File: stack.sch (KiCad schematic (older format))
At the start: 6 parts, among them U26 74LS245, U27 74LS173, U28 74LS173, U29 74LS245, U30 74LS173, U31 74LS173

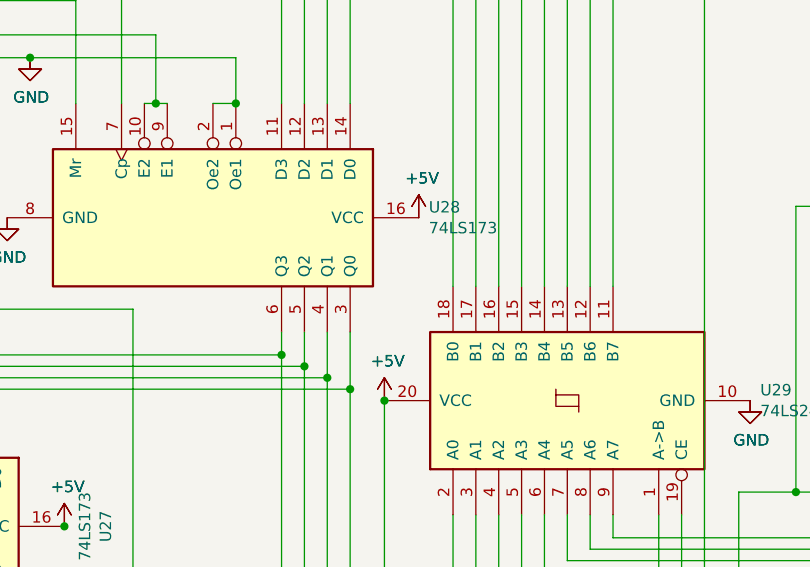
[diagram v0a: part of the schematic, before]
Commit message: fixed more errors
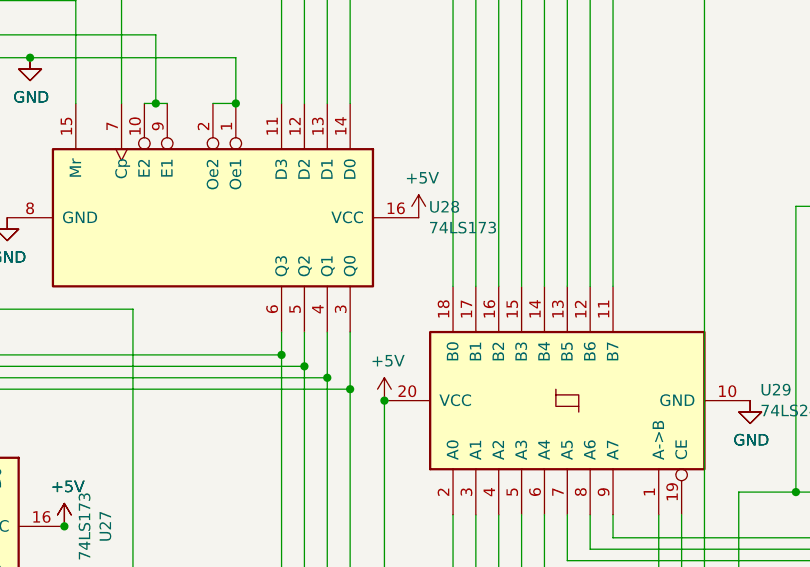
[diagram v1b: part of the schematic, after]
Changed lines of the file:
@@
-$Comp
-L 16bitCpu-rescue:+5V-power #PWR?
-U 1 1 616C3797
-P 5800 4300
-AR Path="/616C3797" Ref="#PWR?"  Part="1"
-AR Path="/5F67C726/616C3797" Ref="#PWR?"  Part="1"
-AR Path="/5F70885A/616C3797" Ref="#PWR?"  Part="1"
-AR Path="/5F733C5E/616C3797" Ref="#PWR?"  Part="1"
-AR Path="/602D4838/616C3797" Ref="#PWR?"  Part="1"
-AR Path="/603B00C8/616C3797" Ref="#PWR?"  Part="1"
-AR Path="/603B766D/616C3797" Ref="#PWR?"  Part="1"
-AR Path="/5F74778C/616C3797" Ref="#PWR?"  Part="1"
-AR Path="/5FB94562/616C3797" Ref="#PWR?"  Part="1"
-AR Path="/61968B9B/616C3797" Ref="#PWR0110"  Part="1"
-F 0 "#PWR0110" H 5800 4150 50  0001 C CNN
-F 1 "+5V" H 5815 4473 50  0000 C CNN
-F 2 "" H 5800 4300 50  0001 C CNN
-F 3 "" H 5800 4300 50  0001 C CNN
-	1    5800 4300
-	1    0    0    -1
-$EndComp
 $Comp
 L 16bitCpu-rescue:+5V-power #PWR?
@@
 	1    0    0    -1
 $EndComp
-$Comp
-L 16bitCpu-rescue:+5V-power #PWR?
-U 1 1 616C379A
-P 5950 3500
-AR Path="/616C379A" Ref="#PWR?"  Part="1"
-AR Path="/5F67C726/616C379A" Ref="#PWR?"  Part="1"
-AR Path="/5F70885A/616C379A" Ref="#PWR?"  Part="1"
-AR Path="/5F733C5E/616C379A" Ref="#PWR?"  Part="1"
-AR Path="/602D4838/616C379A" Ref="#PWR?"  Part="1"
-AR Path="/603B00C8/616C379A" Ref="#PWR?"  Part="1"
-AR Path="/603B766D/616C379A" Ref="#PWR?"  Part="1"
-AR Path="/5F74778C/616C379A" Ref="#PWR?"  Part="1"
-AR Path="/5FB94562/616C379A" Ref="#PWR?"  Part="1"
-AR Path="/61968B9B/616C379A" Ref="#PWR0111"  Part="1"
-F 0 "#PWR0111" H 5950 3350 50  0001 C CNN
-F 1 "+5V" H 5965 3673 50  0000 C CNN
-F 2 "" H 5950 3500 50  0001 C CNN
-F 3 "" H 5950 3500 50  0001 C CNN
-	1    5950 3500
-	1    0    0    -1
-$EndComp
